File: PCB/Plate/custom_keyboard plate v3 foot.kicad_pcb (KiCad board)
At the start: 2 copper layers, 20 x 99.5 mm, 2 parts, among them M3 MountingHole_3.2mm_M3

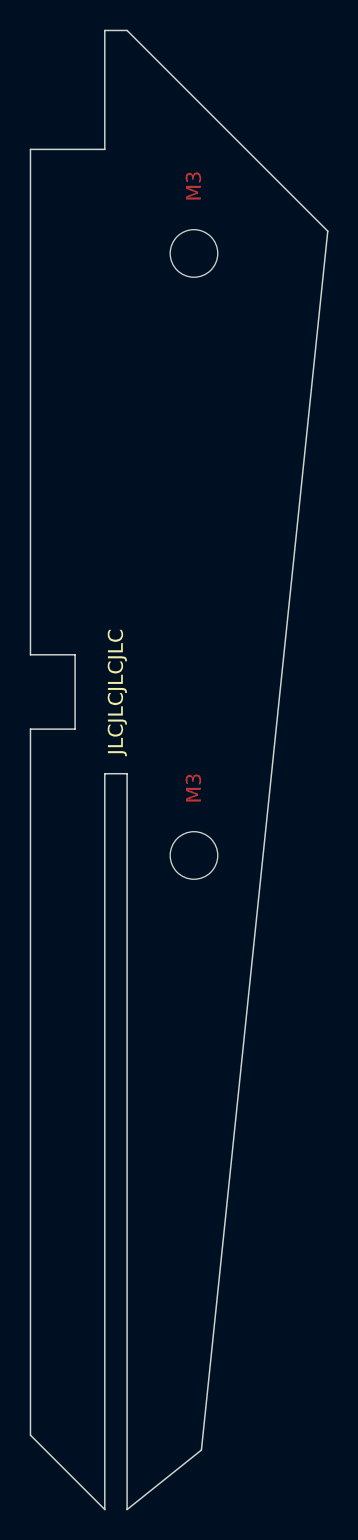
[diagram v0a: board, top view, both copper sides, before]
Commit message: Final verification before ordering
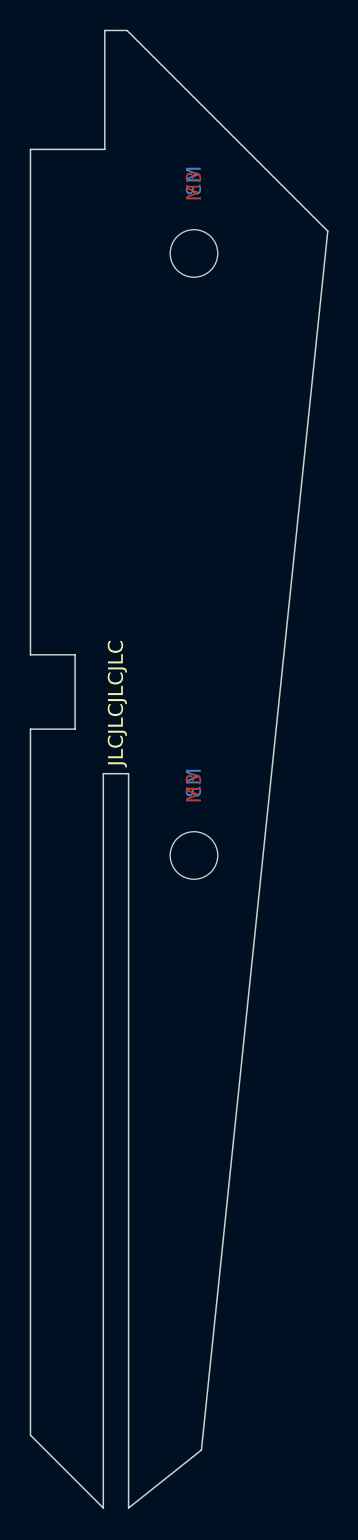
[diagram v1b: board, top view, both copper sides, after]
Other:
- board size 20 x 99.5 mm -> 20 x 99.4 mm
- board text added: "© 2022 Howard Tseng"
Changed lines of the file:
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@@
     (thickness 1.6)
   )
-  (paper "A4")
+  (paper "A3")
   (layers
     (0 "F.Cu" signal)
@@
   )
   (setup
+    (stackup
+      (layer "F.SilkS" (type "Top Silk Screen"))
+      (layer "F.Paste" (type "Top Solder Paste"))
+      (layer "F.Mask" (type "Top Solder Mask") (thickness 0.01))
+      (layer "F.Cu" (type "copper") (thickness 0.035))
+      (layer "dielectric 1" (type "core") (thickness 1.51) (material "FR4") (epsilon_r 4.5) (loss_tangent 0.02))
+      (layer "B.Cu" (type "copper") (thickness 0.035))
+      (layer "B.Mask" (type "Bottom Solder Mask") (thickness 0.01))
+      (layer "B.Paste" (type "Bottom Solder Paste"))
+      (layer "B.SilkS" (type "Bottom Silk Screen"))
+      (layer "F.SilkS" (type "Top Silk Screen"))
+      (layer "F.Paste" (type "Top Solder Paste"))
+      (layer "F.Mask" (type "Top Solder Mask") (thickness 0.01))
+      (layer "F.Cu" (type "copper") (thickness 0.035))
+      (layer "dielectric 2" (type "core") (thickness 1.51) (material "FR4") (epsilon_r 4.5) (loss_tangent 0.02))
+      (layer "B.Cu" (type "copper") (thickness 0.035))
+      (layer "B.Mask" (type "Bottom Solder Mask") (thickness 0.01))
+      (layer "B.Paste" (type "Bottom Solder Paste"))
+      (layer "B.SilkS" (type "Bottom Silk Screen"))
+      (layer "F.SilkS" (type "Top Silk Screen"))
+      (layer "F.Paste" (type "Top Solder Paste"))
+      (layer "F.Mask" (type "Top Solder Mask") (thickness 0.01))
+      (layer "F.Cu" (type "copper") (thickness 0.035))
+      (layer "dielectric 3" (type "core") (thickness 1.51) (material "FR4") (epsilon_r 4.5) (loss_tangent 0.02))
+      (layer "B.Cu" (type "copper") (thickness 0.035))
+      (layer "B.Mask" (type "Bottom Solder Mask") (thickness 0.01))
+      (layer "B.Paste" (type "Bottom Solder Paste"))
+      (layer "B.SilkS" (type "Bottom Silk Screen"))
+      (layer "F.SilkS" (type "Top Silk Screen"))
+      (layer "F.Paste" (type "Top Solder Paste"))
+      (layer "F.Mask" (type "Top Solder Mask") (thickness 0.01))
+      (layer "F.Cu" (type "copper") (thickness 0.035))
+      (layer "dielectric 4" (type "core") (thickness 1.51) (material "FR4") (epsilon_r 4.5) (loss_tangent 0.02))
+      (layer "B.Cu" (type "copper") (thickness 0.035))
+      (layer "B.Mask" (type "Bottom Solder Mask") (thickness 0.01))
+      (layer "B.Paste" (type "Bottom Solder Paste"))
+      (layer "B.SilkS" (type "Bottom Silk Screen"))
+      (layer "F.SilkS" (type "Top Silk Screen"))
+      (layer "F.Paste" (type "Top Solder Paste"))
+      (layer "F.Mask" (type "Top Solder Mask") (thickness 0.01))
+      (layer "F.Cu" (type "copper") (thickness 0.035))
+      (layer "dielectric 5" (type "core") (thickness 1.51) (material "FR4") (epsilon_r 4.5) (loss_tangent 0.02))
+      (layer "B.Cu" (type "copper") (thickness 0.035))
+      (layer "B.Mask" (type "Bottom Solder Mask") (thickness 0.01))
+      (layer "B.Paste" (type "Bottom Solder Paste"))
+      (layer "B.SilkS" (type "Bottom Silk Screen"))
+      (layer "F.SilkS" (type "Top Silk Screen"))
+      (layer "F.Paste" (type "Top Solder Paste"))
+      (layer "F.Mask" (type "Top Solder Mask") (thickness 0.01))
+      (layer "F.Cu" (type "copper") (thickness 0.035))
+      (layer "dielectric 6" (type "core") (thickness 1.51) (material "FR4") (epsilon_r 4.5) (loss_tangent 0.02))
+      (layer "B.Cu" (type "copper") (thickness 0.035))
+      (layer "B.Mask" (type "Bottom Solder Mask") (thickness 0.01))
+      (layer "B.Paste" (type "Bottom Solder Paste"))
+      (layer "B.SilkS" (type "Bottom Silk Screen"))
+      (layer "F.SilkS" (type "Top Silk Screen"))
+      (layer "F.Paste" (type "Top Solder Paste"))
+      (layer "F.Mask" (type "Top Solder Mask") (thickness 0.01))
+      (layer "F.Cu" (type "copper") (thickness 0.035))
+      (layer "dielectric 7" (type "core") (thickness 1.51) (material "FR4") (epsilon_r 4.5) (loss_tangent 0.02))
+      (layer "B.Cu" (type "copper") (thickness 0.035))
+      (layer "B.Mask" (type "Bottom Solder Mask") (thickness 0.01))
+      (layer "B.Paste" (type "Bottom Solder Paste"))
+      (layer "B.SilkS" (type "Bottom Silk Screen"))
+      (copper_finish "None")
+      (dielectric_constraints no)
+    )
     (pad_to_mask_clearance 0)
+    (grid_origin 211.1242 72.2267)
     (pcbplotparams
       (layerselection 0x00010fc_ffffffff)
@@
       (effects (font (size 1 1) (thickness 0.2)))
     )
+    (fp_text user "${REFERENCE}" (at 0 34.6 90) (layer "B.Cu")
+      (effects (font (size 1 1) (thickness 0.2)) (justify left mirror))
+    )
     (fp_text user "${REFERENCE}" (at 0.3 0) (layer "F.Fab")
       (effects (font (size 1 1) (thickness 0.2)))
@@
       (effects (font (size 1 1) (thickness 0.2)))
     )
+    (fp_text user "${REFERENCE}" (at 0 -46.4 90) (layer "B.Cu")
+      (effects (font (size 1 1) (thickness 0.2)) (justify left mirror))
+    )
     (fp_text user "${REFERENCE}" (at 0.3 0) (layer "F.Fab")
       (effects (font (size 1 1) (thickness 0.2)))
@@
   )
   (gr_line (start 154 42) (end 155.5 42) (layer "Edge.Cuts") (width 0.1))
-  (gr_line (start 155.5 141.5) (end 160.5 137.5) (layer "Edge.Cuts") (width 0.1))
-  (gr_line (start 154 92) (end 155.5 92) (layer "Edge.Cuts") (width 0.1))
+  (gr_line (start 155.6 141.4) (end 160.5 137.5) (layer "Edge.Cuts") (width 0.1))
+  (gr_line (start 153.9 92) (end 155.6 92) (layer "Edge.Cuts") (width 0.1))
   (gr_line (start 154 50) (end 154 42) (layer "Edge.Cuts") (width 0.1))
-  (gr_line (start 154 92) (end 154 141.5) (layer "Edge.Cuts") (width 0.1))
-  (gr_line (start 155.5 141.5) (end 155.5 92) (layer "Edge.Cuts") (width 0.1))
+  (gr_line (start 153.9 92) (end 153.9 141.4) (layer "Edge.Cuts") (width 0.1))
+  (gr_line (start 155.6 141.4) (end 155.6 92) (layer "Edge.Cuts") (width 0.1))
   (gr_line (start 155.5 42) (end 169 55.5) (layer "Edge.Cuts") (width 0.1))
-  (gr_line (start 154 141.5) (end 149 136.5) (layer "Edge.Cuts") (width 0.1))
+  (gr_line (start 153.9 141.4) (end 149 136.5) (layer "Edge.Cuts") (width 0.1))
   (gr_line (start 154 50) (end 149 50) (layer "Edge.Cuts") (width 0.1))
   (gr_line (start 149 84) (end 149 50) (layer "Edge.Cuts") (width 0.1))
@@
   (gr_line (start 152 84) (end 152 89) (layer "Edge.Cuts") (width 0.1))
   (gr_line (start 169 55.5) (end 160.5 137.5) (layer "Edge.Cuts") (width 0.1))
-  (gr_text "JLCJLCJLCJLC" (at 154.75 86.5 90) (layer "F.SilkS")
-    (effects (font (size 1 1) (thickness 0.15)))
+  (gr_text "© 2022 Howard Tseng" (at 154.749781 91.49212 90) (layer "B.SilkS")
+    (effects (font (size 1 1) (thickness 0.15)) (justify right mirror))
+  )
+  (gr_text "JLCJLCJLCJLC" (at 154.75 91.5 90) (layer "F.SilkS")
+    (effects (font (size 1 1) (thickness 0.15)) (justify left))
   )
 )
